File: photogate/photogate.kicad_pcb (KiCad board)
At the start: 2 copper layers, 72.4 x 62.2 mm, 22 parts, among them P2_Jack_F(Leds)1 SJ1-3525N

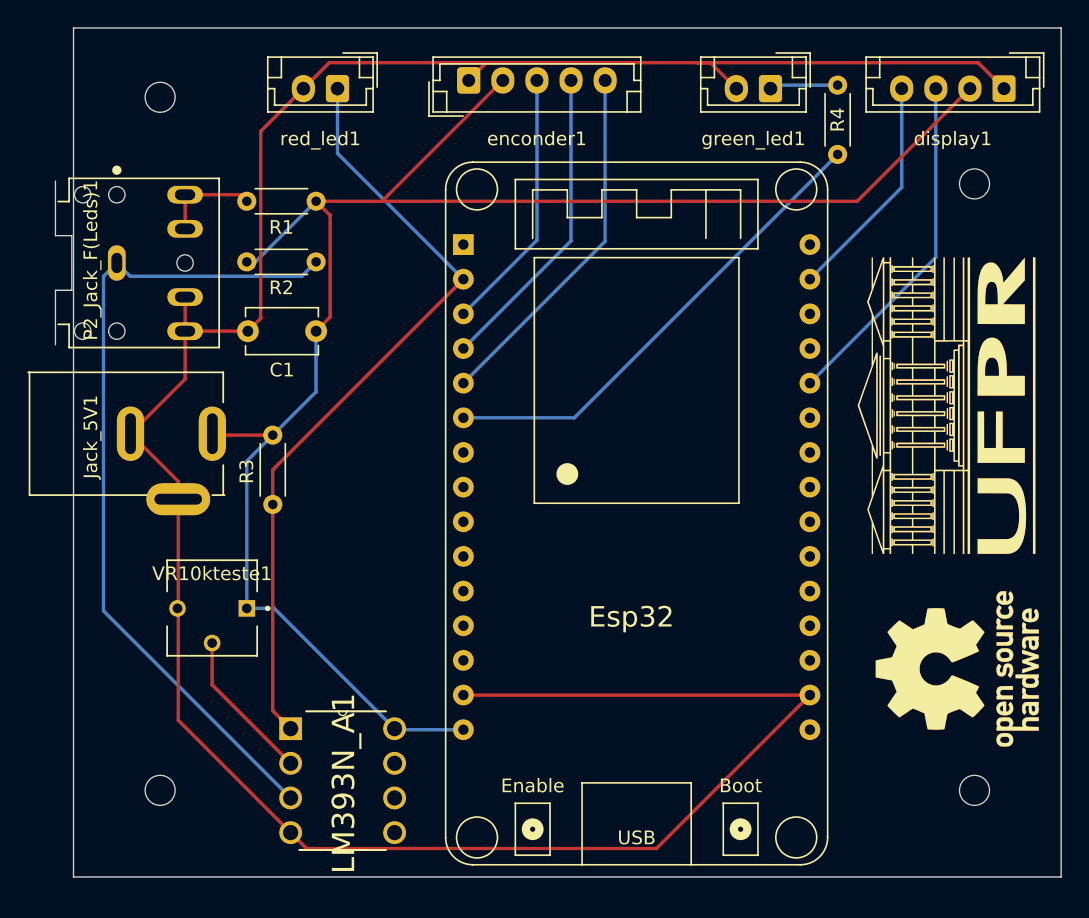
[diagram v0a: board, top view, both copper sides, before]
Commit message: Melhoras na placa
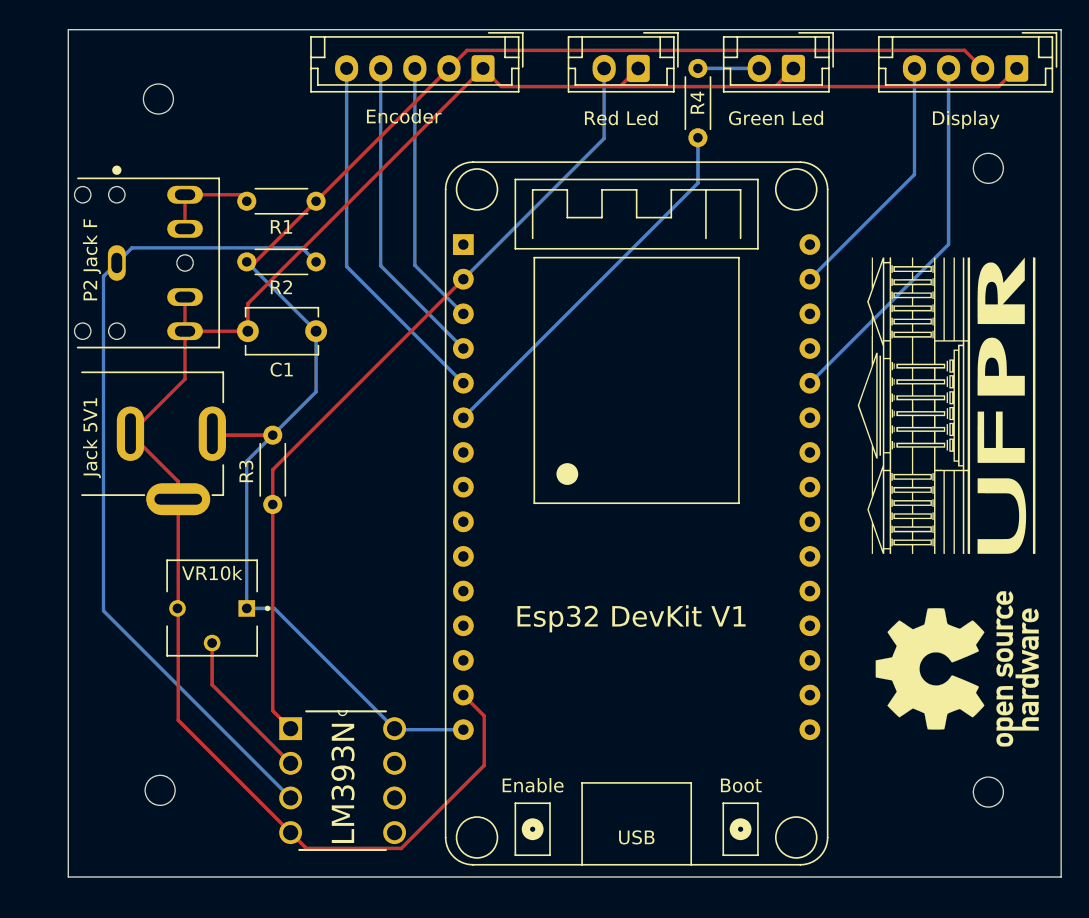
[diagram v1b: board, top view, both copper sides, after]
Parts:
- removed the REF** at (167.3, 111.6)
- removed the REF** at (168.5, 76.1)
- removed the REF** at (168.5, 120.5)
- removed the UFPR at (166.2, 92.1)
- added REF**: MountingHole_2.2mm_M2, MountingHole:MountingHole_2.2mm_M2, F.Cu at (169.5, 74.9)
- added REF**: MountingHole_2.2mm_M2, MountingHole:MountingHole_2.2mm_M2, F.Cu at (169.5, 120.7)
- Esp32 DevKit V1: renamed from Esp32
- Green Led: renamed from green_led1
- Inferior Esquerdo: renamed from REF**
- Jack 5V1: renamed from Jack_5V1
- P2 Jack F: renamed from P2_Jack_F(Leds)1
- Red Led: renamed from red_led1
- moved Red Led 22.1 mm to (143.9, 67.6)
- moved R4 10.3 mm to (148.3, 72.7)
- moved Green Led 2.24 mm to (155.3, 67.6)
- moved Display 1.75 mm to (171.6, 67.6)
- moved Encoder 1.37 mm to (132.5, 67.6), turned to 180 degrees
- moved REF** 0.18 mm to (108.7, 69.8)
- renumbered display1 to Display, enconder1 to Encoder, LM393N_A1 to LM393N, VR10kteste1 to VR10k
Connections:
- Esp32 DevKit V1 pad 17: GND -> unconnected-(Esp32-Pad17)
- Green Led pad 1: /FUNC_LED -> GND
- Green Led pad 2: GND -> /FUNC_LED
- Red Led pad 1: /D0 -> GND
- Red Led pad 2: GND -> /D0
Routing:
- net GND: track 197.9 -> 143.7 mm
- net Net-(C1-Pad1): track 127.6 -> 114.5 mm
- net Net-(Esp32-Pad6): track 35.4 -> 27.6 mm
- net /D0: track 57.1 -> 59.0 mm
- net /SCL: track 16.8 -> 18.6 mm
- net /SDA: track 25.4 -> 27.3 mm
- net /FUNC_LED: track 5.03 -> 4.50 mm
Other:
- board size 72.4 x 62.2 mm -> 72.8 x 62.1 mm
